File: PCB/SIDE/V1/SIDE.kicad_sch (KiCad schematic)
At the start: 21 parts, among them IC1 VEML6030-GS15, J1 pin, J2 pin, J4 SM06B-SRSS-TB(LF)(SN), Q1 PJE8408_R1_00001, Q2 PJE8408_R1_00001, U1 AS7341DLG, U2 TMP112xxDRL, U3 SHT4x

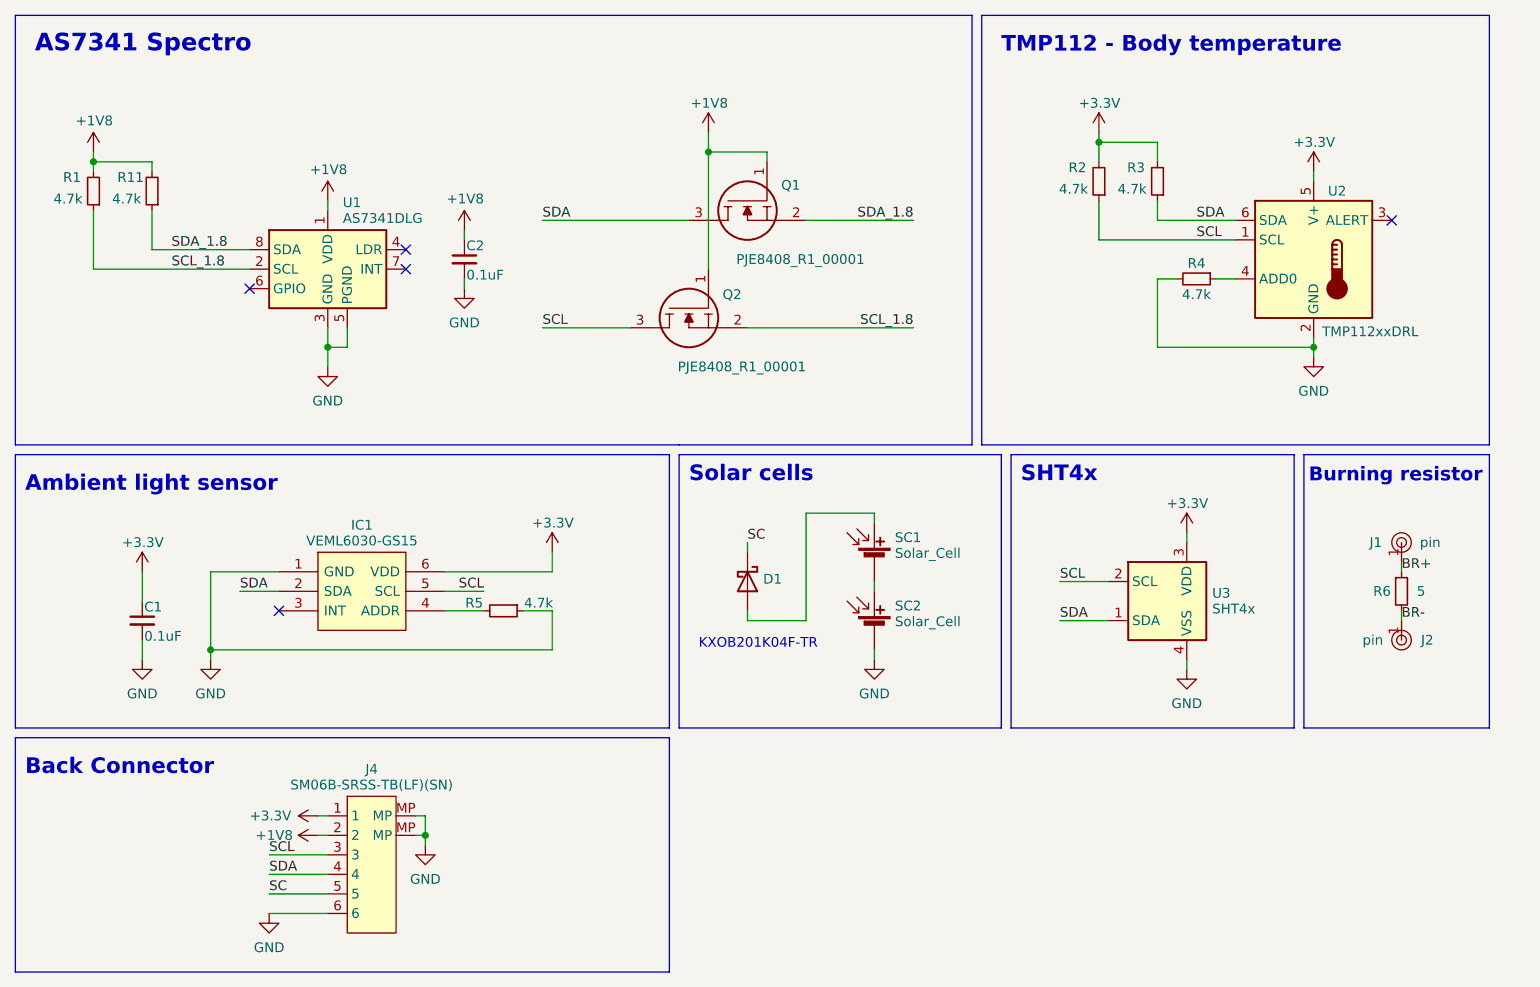
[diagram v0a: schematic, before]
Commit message: udated by FZ
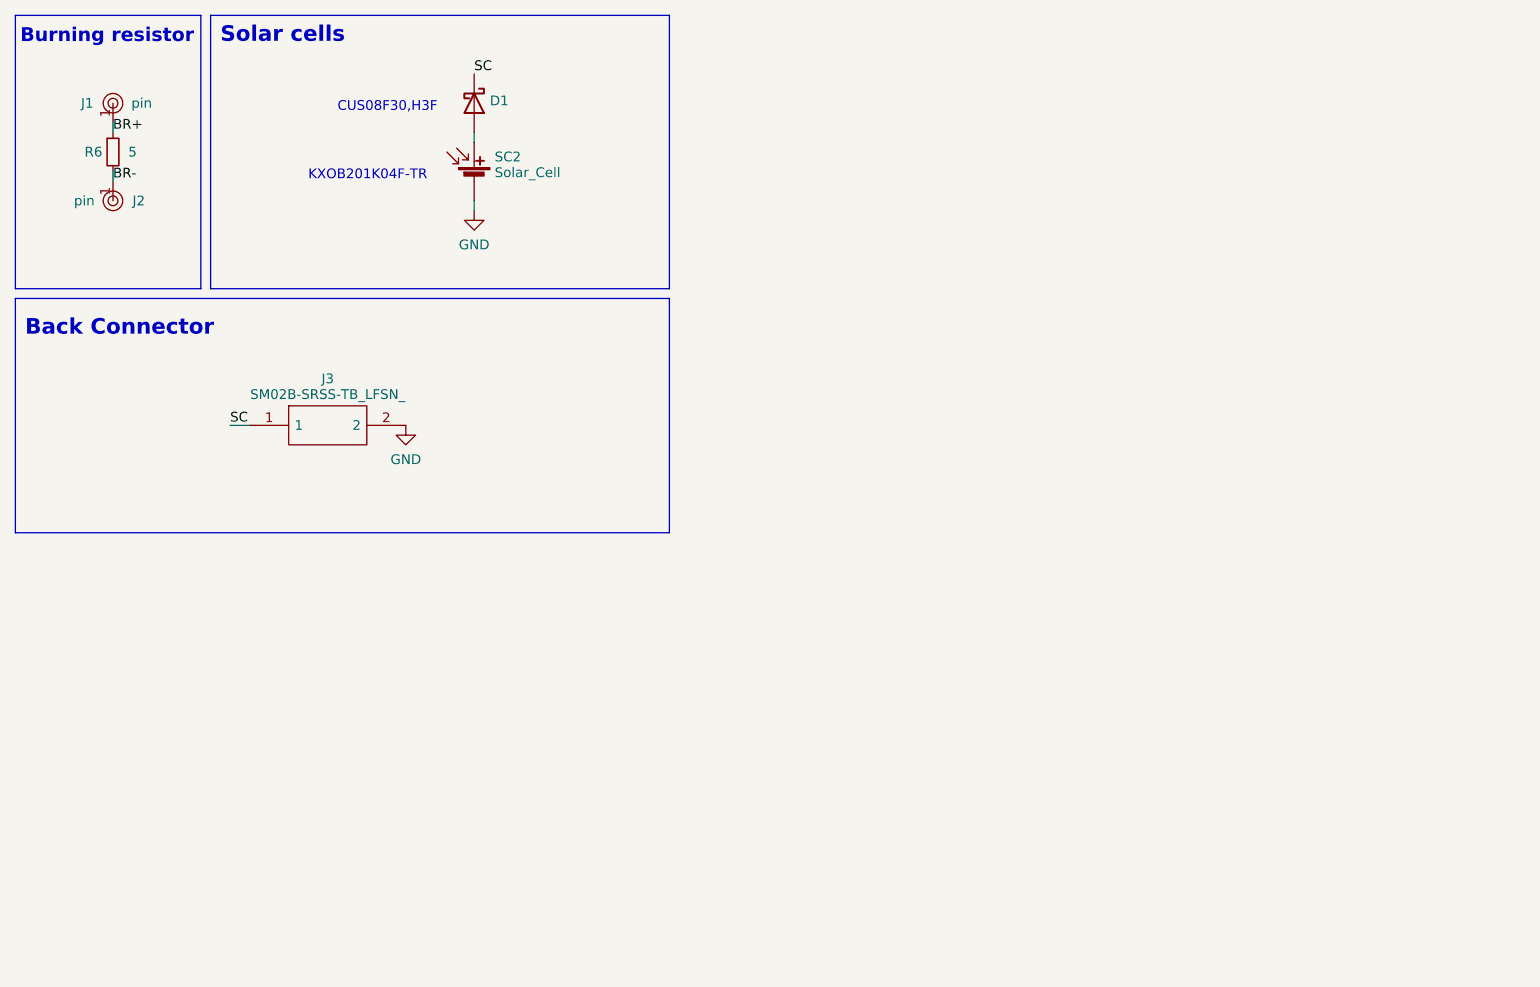
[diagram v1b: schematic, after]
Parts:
- removed C1, C2: 0.1uF, Capacitor_SMD:C_0603_1608Metric_Pad1.08x0.95mm_HandSolder, symbol Device:C_Small
- removed IC1: VEML6030-GS15, SamacSys_Parts:VEML6030GS15, symbol SamacSys_Parts:VEML6030-GS15
- removed J4: SM06B-SRSS-TB(LF)(SN), Connector_JST:JST_SH_SM06B-SRSS-TB_1x06-1MP_P1.00mm_Horizontal, symbol Mylib:BM06B-SURS-TF(LF)(SN)
- removed Q1, Q2: PJE8408_R1_00001, SamacSys_Parts:SOTFL50P160X60-3N, symbol SamacSys_Parts:PJE8408_R1_00001
- removed R1, R11, R2, R3, R4, R5: 4.7k, Resistor_SMD:R_0603_1608Metric_Pad0.98x0.95mm_HandSolder, symbol Device:R_Small
- removed SC1: Solar_Cell, Mylib:KXOB201K04F-TR, symbol Device:Solar_Cell
- removed U1: AS7341DLG, Package_LGA:AMS_OLGA-8_2x3.1mm_P0.8mm, symbol Sensor_Optical:AS7341DLG
- removed U2: TMP112xxDRL, Package_TO_SOT_SMD:SOT-563, symbol Sensor_Temperature:TMP112xxDRL
- removed U3: SHT4x, Sensor_Humidity:Sensirion_DFN-4_1.5x1.5mm_P0.8mm_SHT4x_NoCentralPad, symbol Sensor_Humidity:SHT4x
- added J3: SM02B-SRSS-TB_LFSN_, SM02B-SRSS-TB, symbol SamacSys_Parts:SM02B-SRSS-TB_LFSN_
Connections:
- net GND: now also J3.2
- net SC: now also J3.1
- net at SC2.1 (+): now also D1.2 (A)
- no-connect marks 5 -> 0
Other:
- note added: "CUS08F30,H3F"
- note removed: "AS7341 Spectro"
- note removed: "Ambient light sensor"
- note removed: "SHT4x"
- note removed: "TMP112 - Body temperature"
- moved on the sheet: D1, J1, J2, R6, SC2
